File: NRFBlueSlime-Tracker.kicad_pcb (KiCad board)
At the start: 4 copper layers, 38 x 20 mm, 61 parts, among them J1 GT-USB-7010ASV, Q1 NTS2101PT1G, SW1 TS-1088-AR02016, U1 ICM-45686, U2 E73-2G4M08S1C, U3 LIS2MDL, U4 EA8103DHR, U5 TP4057-42-SOT26-R, X1 S2D32.768KB20F30T, Y1 Q13FC13500004

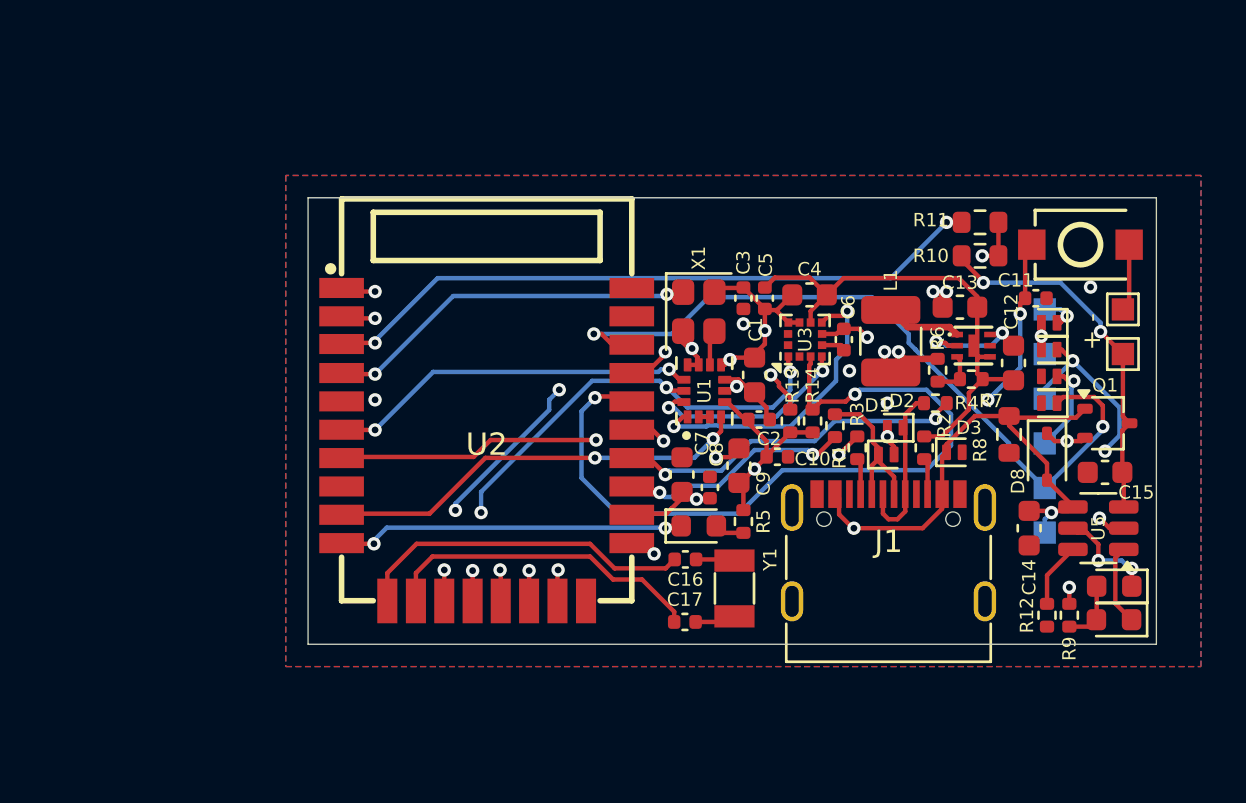
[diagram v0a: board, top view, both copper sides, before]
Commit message: sihashkdasfhjkads
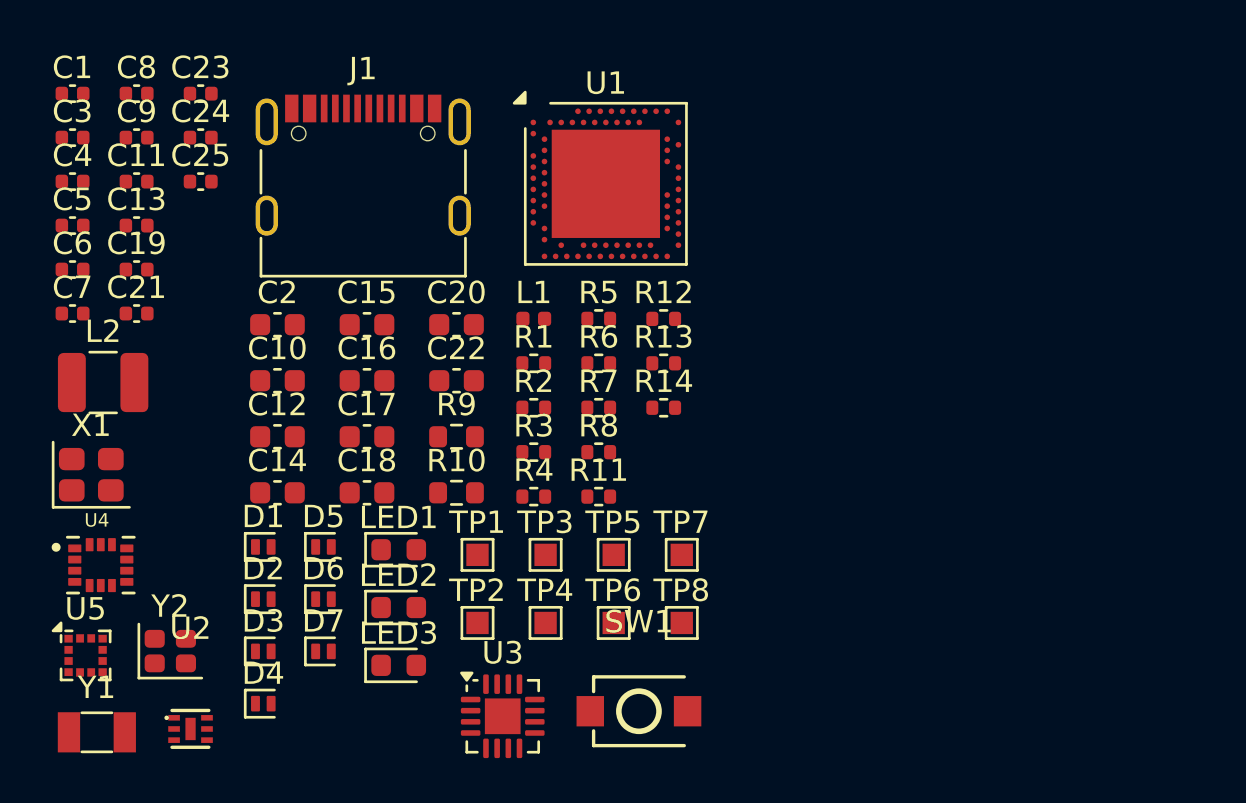
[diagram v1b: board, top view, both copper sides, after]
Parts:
- removed D8: 1N5819WS, Diode_SMD:D_SOD-323
- removed Q1: NTS2101PT1G, Package_TO_SOT_SMD:SOT-323_SC-70
- added C18: 10u, Capacitor_SMD:C_0603_1608Metric, F.Cu at (52.6, 47.2)
- added C19: 100n, Capacitor_SMD:C_0402_1005Metric, F.Cu at (42.3, 37.2)
- added C20: 10u, Capacitor_SMD:C_0603_1608Metric, F.Cu at (56.6, 39.7)
- added C21: 100n, Capacitor_SMD:C_0402_1005Metric, F.Cu at (42.3, 39.2)
- added C22: 10u, Capacitor_SMD:C_0603_1608Metric, F.Cu at (56.6, 42.2)
- added C23: 100n, Capacitor_SMD:C_0402_1005Metric, F.Cu at (45.2, 29.3)
- added C24: 220n, Capacitor_SMD:C_0402_1005Metric, F.Cu at (45.2, 31.3)
- added C25: 220n, Capacitor_SMD:C_0402_1005Metric, F.Cu at (45.2, 33.3)
- added L2: 2.2u, Inductor_SMD:L_1210_3225Metric, F.Cu at (40.8, 42.3)
- added Y2: XL7EL89CKI-111YLC-32M, Crystal:Crystal_SMD_2016-4Pin_2.0x1.6mm, F.Cu at (43.8, 54.3)
- C1: value 10u -> 100p; footprint Capacitor_SMD:C_0603_1608Metric -> Capacitor_SMD:C_0402_1005Metric
- C10, C2: value 100n -> 1u; footprint Capacitor_SMD:C_0402_1005Metric -> Capacitor_SMD:C_0603_1608Metric
- C11, C6: value 220n -> 100n
- C12: value 10u -> 1u
- C13: value 10u -> 100n; footprint Capacitor_SMD:C_0603_1608Metric -> Capacitor_SMD:C_0402_1005Metric
- C14: value 1u -> 10u
- C16, C17: value 22p -> 4.7u; footprint Capacitor_SMD:C_0402_1005Metric -> Capacitor_SMD:C_0603_1608Metric
- C3: value 100n -> 100p
- C4: value 10u -> 15p; footprint Capacitor_SMD:C_0603_1608Metric -> Capacitor_SMD:C_0402_1005Metric
- C5: value 100n -> 15p
- C7: value 1u -> 0.8p; footprint Capacitor_SMD:C_0603_1608Metric -> Capacitor_SMD:C_0402_1005Metric
- C8: value 100n -> 6.8p
- C9: value 1u -> 6.8p; footprint Capacitor_SMD:C_0603_1608Metric -> Capacitor_SMD:C_0402_1005Metric
- L1: value 2.2u -> 4.7n; footprint Inductor_SMD:L_1210_3225Metric -> Inductor_SMD:L_0402_1005Metric
- R1, R2: value 5.1k -> 27
- R10: value 100k -> 51k
- R11: value 51k -> 10k; footprint Resistor_SMD:R_0603_1608Metric -> Resistor_SMD:R_0402_1005Metric
- R3: value 27 -> 1k
- R4: value 27 -> 5.1k
- R5: value 1k -> 5.1k
- R8: value 100k -> 10k; footprint Resistor_SMD:R_0603_1608Metric -> Resistor_SMD:R_0402_1005Metric
- R9: value 1k -> 100k; footprint Resistor_SMD:R_0402_1005Metric -> Resistor_SMD:R_0603_1608Metric
- TP1, TP2, TP3, TP4, TP5, TP6: moved to F.Cu
- U1: value ICM-45686 -> nRF52840; footprint 42688:PQFN50P300X250X97-14N -> Package_DFN_QFN:Nordic_AQFN-73-1EP_7x7mm_P0.5mm
- U2: value E73-2G4M08S1C -> EA8103DHR; footprint nrf:E73-2G4M08S1C_nobottom -> nrfslime:DFN-6_L1.5-W1.5-P0.50-BL-EP1.0
- U3: value LIS2MDL -> BQ24075RGT; footprint Package_LGA:LGA-12_2x2mm_P0.5mm -> Package_DFN_QFN:VQFN-16-1EP_3x3mm_P0.5mm_EP1.6x1.6mm
- U4: value EA8103DHR -> ICM-45686; footprint nrfslime:DFN-6_L1.5-W1.5-P0.50-BL-EP1.0 -> 42688:PQFN50P300X250X97-14N
- U5: value TP4057-42-SOT26-R -> LIS2MDL; footprint Package_TO_SOT_SMD:SOT-23-6 -> Package_LGA:LGA-12_2x2mm_P0.5mm
- Y1: value Q13FC13500004 -> XKXGI-SUA-32.768K
- moved U5 45.7 mm to (40.0, 54.5), turned to 0 degrees
- moved C11 40.6 mm to (42.3, 33.3)
- moved U4 40.3 mm to (40.7, 50.5)
- moved D4 38.1 mm to (48.0, 56.7), turned to 0 degrees
- moved C13 37.1 mm to (42.3, 35.2)
- moved D7 35.7 mm to (50.7, 54.3), turned to 0 degrees
- moved C6 34.7 mm to (39.4, 37.2), turned to 0 degrees
- moved D6 34.4 mm to (50.7, 52.0), turned to 0 degrees
- moved C15 33.7 mm to (52.6, 39.7), turned to 0 degrees
- moved C14 33.7 mm to (48.6, 47.2), turned to 0 degrees
- moved C4 33.4 mm to (39.4, 33.3)
- moved D5 33.1 mm to (50.7, 49.6), turned to 0 degrees
- moved C12 33.1 mm to (48.6, 44.7), turned to 0 degrees
- moved C1 33.0 mm to (39.4, 29.3), turned to 0 degrees
- moved LED3 32.2 mm to (54.1, 54.9), turned to 0 degrees
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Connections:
- C1 pad 1: +3V3 -> GND
- C1 pad 2: GND -> Net-(U1-DEC4)
- C10 pad 1: +3V3 -> VBUS
- C11 pad 1: KEY -> VBUS
- C12 pad 1: VDC -> +3V3
- C14 pad 1: GND -> VDC
- C14 pad 2: VBUS -> GND
- C15 pad 1: +BATT -> +3V3
- C16 pad 1: Net-(U2-XL1) -> GND
- C16 pad 2: Net-(C16-Pad2) -> VBUS
- C17 pad 1: Net-(U2-XL2) -> GND
- C17 pad 2: Net-(C17-Pad2) -> Net-(LED2-A)
- C2 pad 1: +3V3 -> GND
- C2 pad 2: GND -> Net-(U1-DEC4)
- C3 pad 1: +3V3 -> GND
- C3 pad 2: GND -> Net-(U1-DEC3)
- C4 pad 1: +3V3 -> Net-(U1-XL1/P0.00)
- C4 pad 2: GND -> Net-(C4-Pad2)
- C5 pad 1: +3V3 -> Net-(U1-XL2/P0.01)
- C5 pad 2: GND -> Net-(C5-Pad2)
- C6 pad 1: Net-(U3-C1) -> GND
- C6 pad 2: GND -> Net-(U1-DEC1)
- C7 pad 1: VBUS -> GND
- C7 pad 2: GND -> Net-(U1-ANT)
- C8 pad 1: VBUS -> Net-(C8-Pad1)
- C8 pad 2: GND -> Net-(U1-XC1)
- C9 pad 1: +3V3 -> Net-(C9-Pad1)
- C9 pad 2: GND -> Net-(U1-XC2)
- D6 pad 1: ~{RST} -> DOCK
- D7 pad 1: DOCK -> ~{RST}
- L1 pad 1: Net-(U4-SW) -> unconnected-(L1-Pad1)
- L1 pad 2: +3V3 -> Net-(U1-ANT)
- R1 pad 1: Net-(J1-CC1) -> DN
- R1 pad 2: GND -> Net-(U1-D-)
- R10 pad 1: BATLVL -> ~{ADC_EN}
- R10 pad 2: +BATT -> BATLVL
- R11 pad 1: ~{ADC_EN} -> Net-(U3-ISET)
- R11 pad 2: BATLVL -> GND
- R12 pad 1: GND -> Net-(U3-TS)
- R12 pad 2: Net-(U5-PROG) -> GND
- R2 pad 1: Net-(J1-CC2) -> DP
- R2 pad 2: GND -> Net-(U1-D+)
- R3 pad 1: DN -> Net-(LED1-A)
- R3 pad 2: Net-(U2-D-) -> +3V3
- R4 pad 1: DP -> Net-(J1-CC1)
- R4 pad 2: Net-(U2-D+) -> GND
- R5 pad 1: Net-(LED1-A) -> Net-(J1-CC2)
- R5 pad 2: +3V3 -> GND
- R6 pad 2: Net-(U4-FB) -> Net-(U2-FB)
- R7 pad 1: Net-(U4-FB) -> Net-(U2-FB)
- R8 pad 1: GND -> Net-(LED2-A)
- R8 pad 2: VBUS -> VDC
- R9 pad 1: Net-(LED2-A) -> BATLVL
- R9 pad 2: VBUS -> +BATT
- U2 pad 1: MOSI -> Net-(U2-SW)
- U2 pad 2: MISO -> VDC
- U2 pad 3: ~{ADC_EN} -> Net-(U2-FB)
- U2 pad 4: OSC_EN -> GND
- U2 pad 5: GND -> unconnected-(U2-NC-Pad5)
- U2 pad 6: ~{CS}_IMU -> VDC
- U2 pad 7: DOCK -> GND
- U3 pad 1: SCLK -> Net-(U3-TS)
- U3 pad 10: +3V3 -> VDC
- U3 pad 11: unconnected-(U3-NC-Pad11) -> VDC
- U3 pad 2: unconnected-(U3-NC-Pad2) -> +BATT
- U3 pad 3: ~{CS}_MAG -> +BATT
- U3 pad 4: MOSI -> GND
- U3 pad 5: Net-(U3-C1) -> GND
- U3 pad 6: GND -> VDC
- U3 pad 7: MISO -> Net-(LED2-K)
- U3 pad 9: +3V3 -> Net-(LED3-K)
- U4 pad 1: Net-(U4-SW) -> MISO
- U4 pad 2: VDC -> GND
- U4 pad 3: Net-(U4-FB) -> GND
- U4 pad 4: GND -> INT
- U4 pad 5: unconnected-(U4-NC-Pad5) -> +3V3
- U4 pad 6: VDC -> GND
- U5 pad 1: Net-(LED2-K) -> SCLK
- U5 pad 2: GND -> unconnected-(U5-NC-Pad2)
- U5 pad 3: +BATT -> ~{CS}_MAG
- U5 pad 4: VBUS -> MOSI
- U5 pad 5: Net-(LED3-K) -> Net-(U5-C1)
- U5 pad 6: Net-(U5-PROG) -> GND
- Y1 pad 1: Net-(C16-Pad2) -> Net-(C4-Pad2)
- Y1 pad 2: Net-(C17-Pad2) -> Net-(C5-Pad2)
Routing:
- net DOCK: track 41.8 -> 0.00 mm, vias 2 -> 0
- net VBUS: track 41.1 -> 0.00 mm, vias 4 -> 0
- net GND: track 39.8 -> 0.00 mm, vias 14 -> 0
- net BATLVL: track 35.2 -> 0.00 mm, vias 4 -> 0
- net ~{CS}_MAG: track 35.0 -> 0.00 mm, vias 2 -> 0
- net SWC: track 33.9 -> 0.00 mm, vias 2 -> 0
- net ~{RST}: track 31.7 -> 0.00 mm, vias 3 -> 0
- net MISO: track 30.5 -> 0.00 mm, vias 3 -> 0
- net ~{ADC_EN}: track 30.1 -> 0.00 mm, vias 2 -> 0
- net +3V3: track 26.7 -> 0.00 mm, vias 9 -> 0
- net MOSI: track 26.2 -> 0.00 mm, vias 3 -> 0
- net SWD: track 25.8 -> 0.00 mm, vias 2 -> 0
- net KEY: track 25.6 -> 0.00 mm, vias 3 -> 0
- net SCLK: track 24.1 -> 0.00 mm, vias 4 -> 0
- net ~{CS}_IMU: track 23.7 -> 0.00 mm, vias 3 -> 0
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- removed copper zone on In2.Cu, net +3V3
- removed copper zone on B.Cu, net GND
- removed copper zone on F.Cu, net GND
- removed copper zone on In1.Cu, net GND
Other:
- board outline removed
- board text removed: "+ -"
